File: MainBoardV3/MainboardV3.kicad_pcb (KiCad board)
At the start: 2 copper layers, 100 x 100 mm, 53 parts, among them J1 Conn_01x02, J10 Conn_01x04, J11 Conn_01x02, J12 Conn_01x02, J13 Conn_01x02, J14 Conn_01x02, J15 Conn_01x02, J16 Conn_01x02, J17 Conn_01x02, J18 Conn_01x03, J19 Conn_02x03_Odd_Even, J2 Conn_01x04, J20 Conn_02x03_Odd_Even, J21 Conn_02x03_Odd_Even, J22 Conn_01x03, J23 Conn_01x05, J24 Conn_02x05_Odd_Even, J3 Conn_01x03, J4 Conn_01x04, J5 Conn_01x05, J6 Conn_01x02, J7 Conn_01x04, J8 Conn_01x04, J9 Conn_01x04, U1 TSR_2-2450, U2 ESP32-S3-DevKitC, U3 TSR_2-2433, U4 TEN_50-2411WI

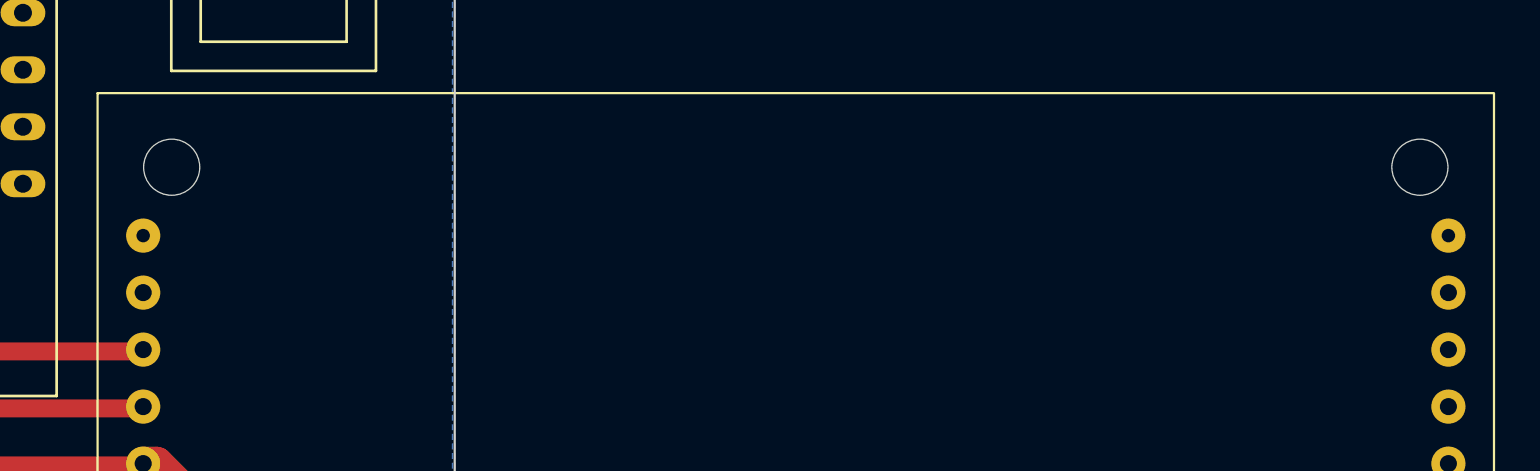
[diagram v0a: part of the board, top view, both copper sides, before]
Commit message: test
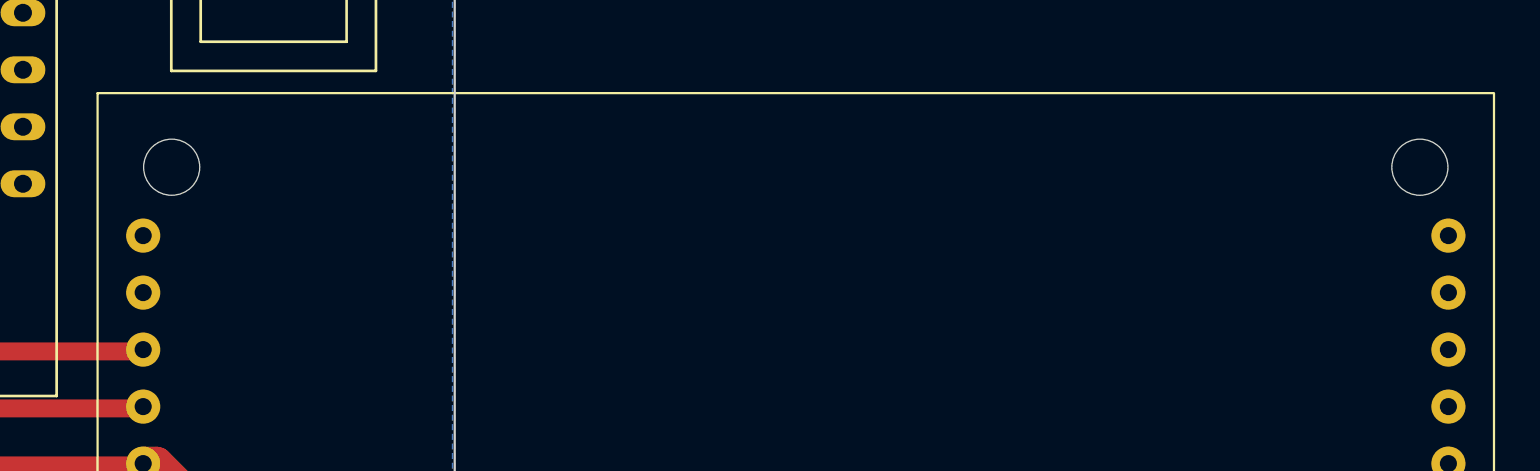
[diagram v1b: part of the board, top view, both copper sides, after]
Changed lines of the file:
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@@
     (pad "" np_thru_hole circle (at 27.813 -9.398) (size 1.524 1.524) (drill 2.5) (layers "F&B.Cu" "*.Mask"))
     (pad "" np_thru_hole circle (at 27.813 9.398) (size 1.524 1.524) (drill 2.5) (layers "F&B.Cu" "*.Mask"))
-    (pad "0" thru_hole circle (at -29.083 -6.35) (size 1.524 1.524) (drill 0.6) (layers "*.Cu" "*.Mask")
+    (pad "0" thru_hole circle (at -29.083 -6.35) (size 1.524 1.524) (drill 0.762) (layers "*.Cu" "*.Mask")
       (net 1 "GND") (pinfunction "GND") (pintype "input"))
-    (pad "0" thru_hole circle (at 29.083 -6.35) (size 1.524 1.524) (drill 0.6) (layers "*.Cu" "*.Mask")
+    (pad "0" thru_hole circle (at 29.083 -6.35) (size 1.524 1.524) (drill 0.762) (layers "*.Cu" "*.Mask")
       (net 1 "GND") (pinfunction "GND") (pintype "input"))
     (pad "1" thru_hole circle (at -29.083 -3.81) (size 1.524 1.524) (drill 0.762) (layers "*.Cu" "*.Mask")
